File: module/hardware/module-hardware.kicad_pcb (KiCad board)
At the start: 4 copper layers, 45.7 x 125.7 mm, 96 parts, among them J1 USB_B_Micro, J10 Conn_01x03, J11 Conn_01x03, J12 Conn_01x03, J13 0, J2 40Pin 0.1", J3 Conn_01x02_Male, J4 40Pin 0.1", J5 Conn_01x03_Male, J6 Conn_01x03_Male, J7 Conn_01x03, J8 Conn_01x03, J9 Conn_01x05_Male, SW1 SW_Push, SW2 SW_Push, U1 NCP1117-3.3_TO252, U2 NCP1117-3.3_TO252, U3 OPA340UA, U4 74LVC2G53, U5 MAX6070, U6 MAX5206, U7 OPA340UA, U8 W25Q128JVS, U9 RP2040, Y1 12MHz 18pF

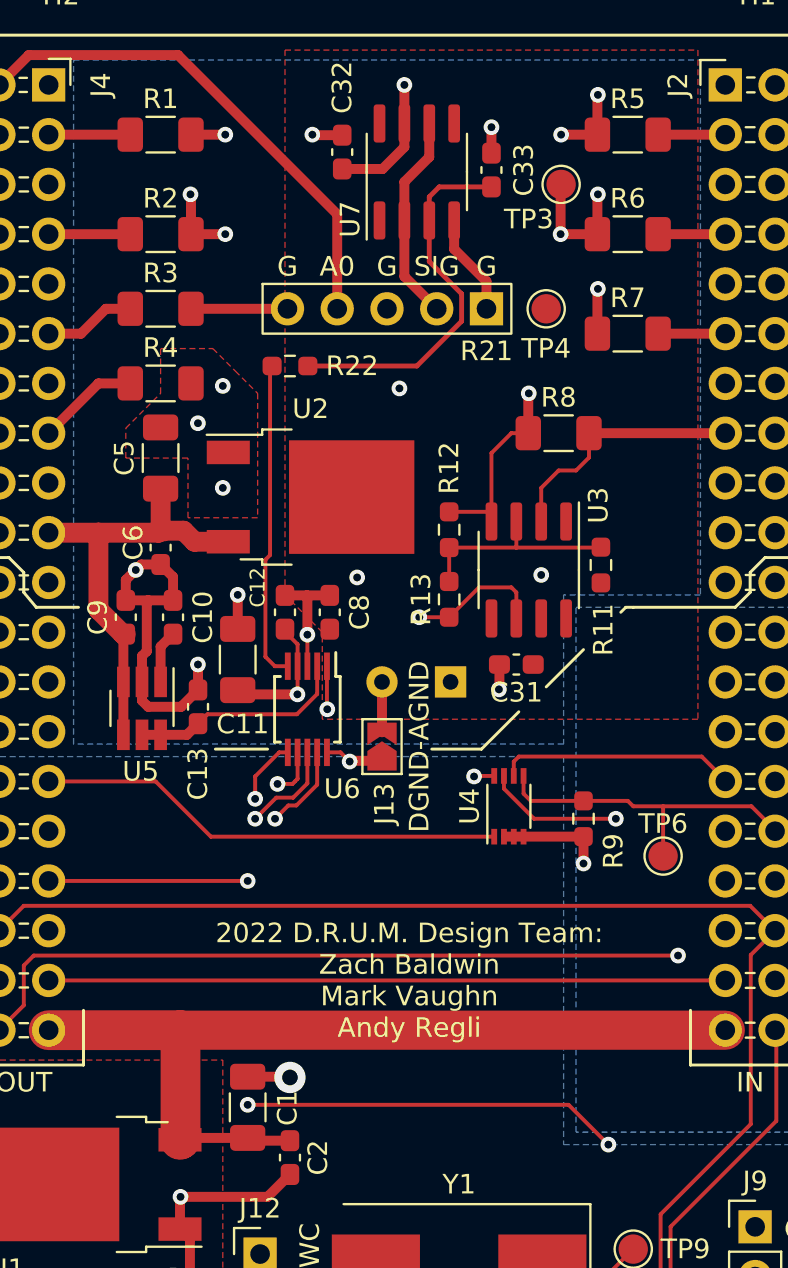
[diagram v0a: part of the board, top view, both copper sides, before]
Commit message: Export Gerbers
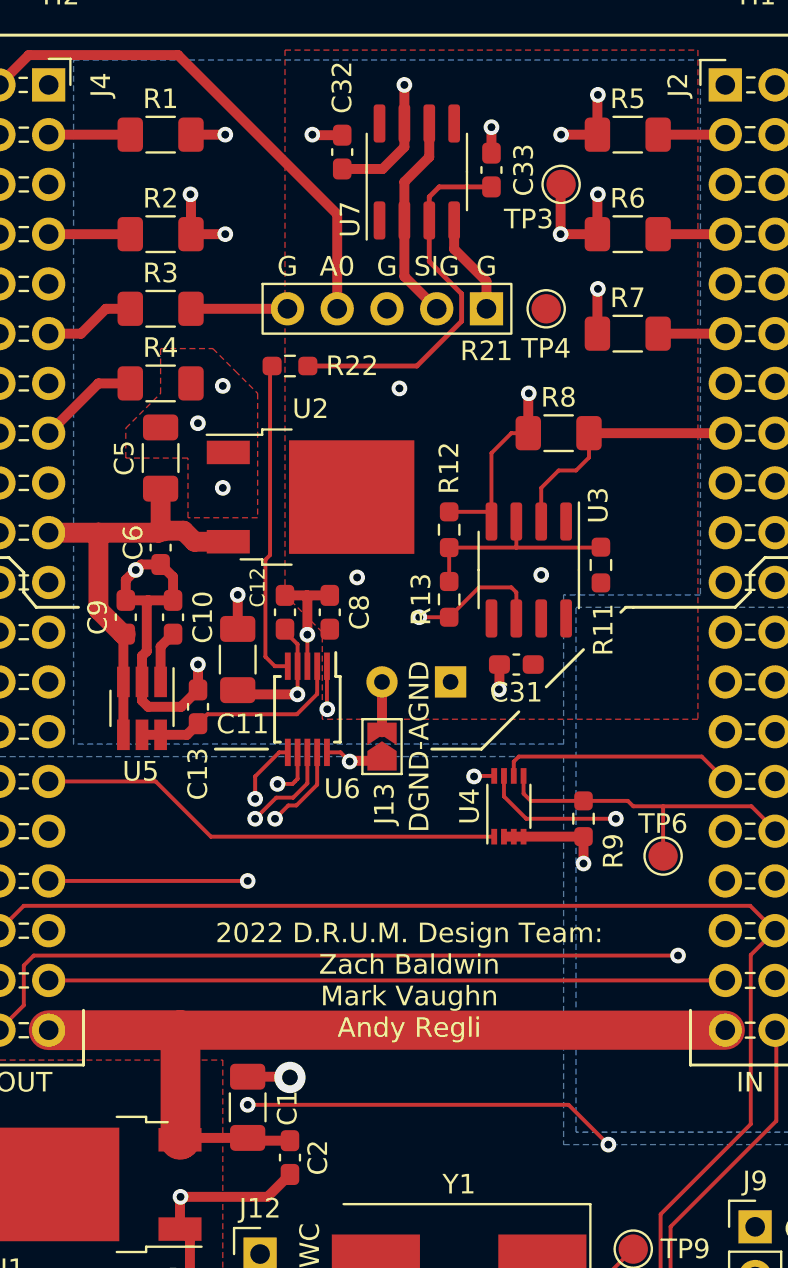
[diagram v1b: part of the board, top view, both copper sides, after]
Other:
- rule pad_to_mask_clearance: 0.05 -> 0
